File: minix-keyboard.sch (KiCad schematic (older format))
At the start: 126 parts, among them J1 AVR-ISP-6, SW1 SW_Push, U1 ATmega32U4-AU, U2 PRTR5V0U2X, Y1 16MHz

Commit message: Add promicro header
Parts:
- added U3: ProMicro-keebio, Keebio-Parts:ArduinoProMicro-TopSide, symbol cookpad-pad-rescue:ProMicro-keebio
- MX1, MX10, MX11, MX12, MX13, MX14, MX15, MX16, MX17, MX18, MX19, MX2, MX20, MX21, MX22, MX23, MX24, MX25, MX26, MX27, MX28, MX29, MX3, MX30, MX31, MX32, MX33, MX34, MX35, MX36, MX37, MX38, MX39, MX4, MX40, MX41, MX42, MX43, MX44, MX45, MX46, MX47, MX48, MX49, MX5, MX50, MX51, MX52, MX53, MX6, MX7, MX8, MX9: symbol MX_Alps_Hybrid:MX-NoLED -> minix-keyboard-rescue:MX-NoLED-MX_Alps_Hybrid
- U2: symbol random-keyboard-parts:PRTR5V0U2X -> minix-keyboard-rescue:PRTR5V0U2X-random-keyboard-parts
- USB1: symbol Type-C:HRO-TYPE-C-31-M-12 -> minix-keyboard-rescue:HRO-TYPE-C-31-M-12-Type-C
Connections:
- net MISO is gone; now on net COL10: J1.1 (MISO), U1.11 (PB3)
- net MOSI is gone; now on net COL11: J1.4 (MOSI), U1.10 (PB2)
- net SCK is gone; now on net COL9: J1.3 (SCK), U1.9 (PB1)
- net COL0: now also U1.25 (PD4), U3.7 (4/PD4)
- net COL1: now also U1.31 (PC6), U3.8 (5/PC6)
- net COL10: now also U3.15 (14/PB3)
- net COL11: now also U3.14 (16/PB2)
- net COL12: now also U1.30 (PB6), U3.13 (10/PB6)
- net COL2: now also U1.27 (PD7), U3.9 (6/PD7)
- net COL3: now also U1.1 (PE6), U3.10 (7/PE6)
- net COL4: now also U1.28 (PB4), U3.11 (8/PB4)
- net COL5: now also U1.29 (PB5), U3.12 (9/PB5)
- net COL6: now also U1.38 (PF5), U3.19 (A2/PF5)
- net COL7: now also U1.37 (PF6), U3.18 (A1/PF6)
- net COL8: now also U1.36 (PF7), U3.17 (A0/PF7)
- net COL9: now also U3.16 (15/PB1)
- net ROW0: now also U1.18 (PD0), U3.6 (3/PD0)
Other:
- note added: "ProMicro"

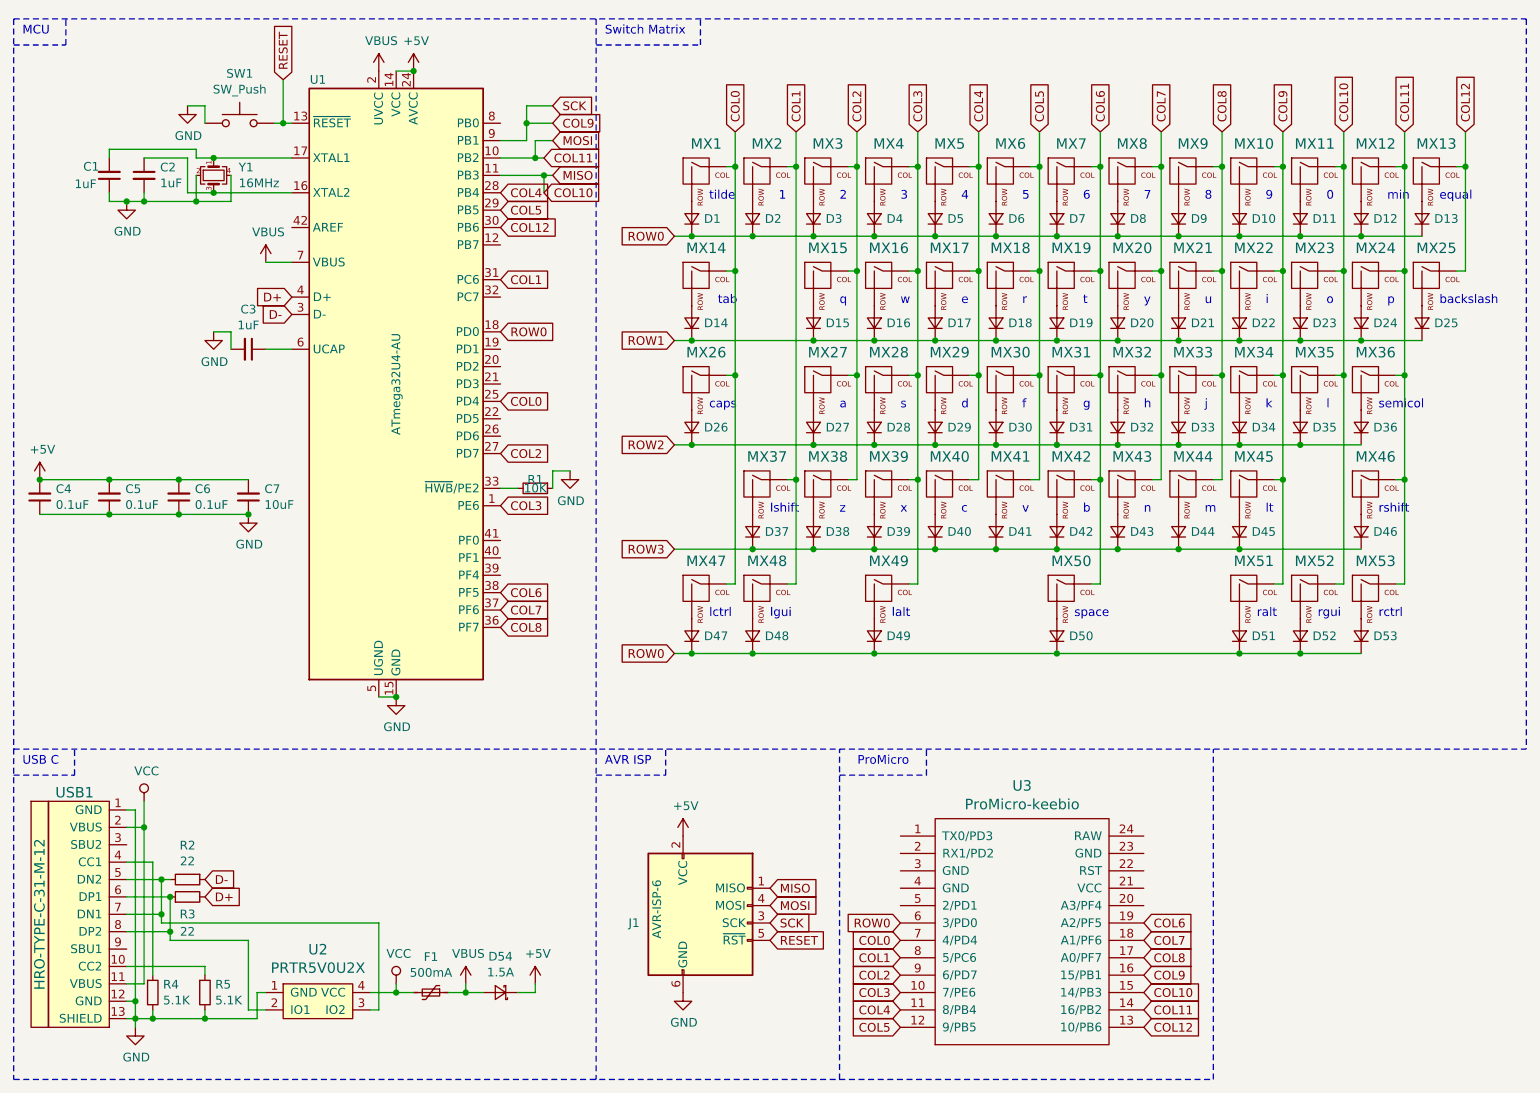
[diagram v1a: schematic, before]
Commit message: Update schematic
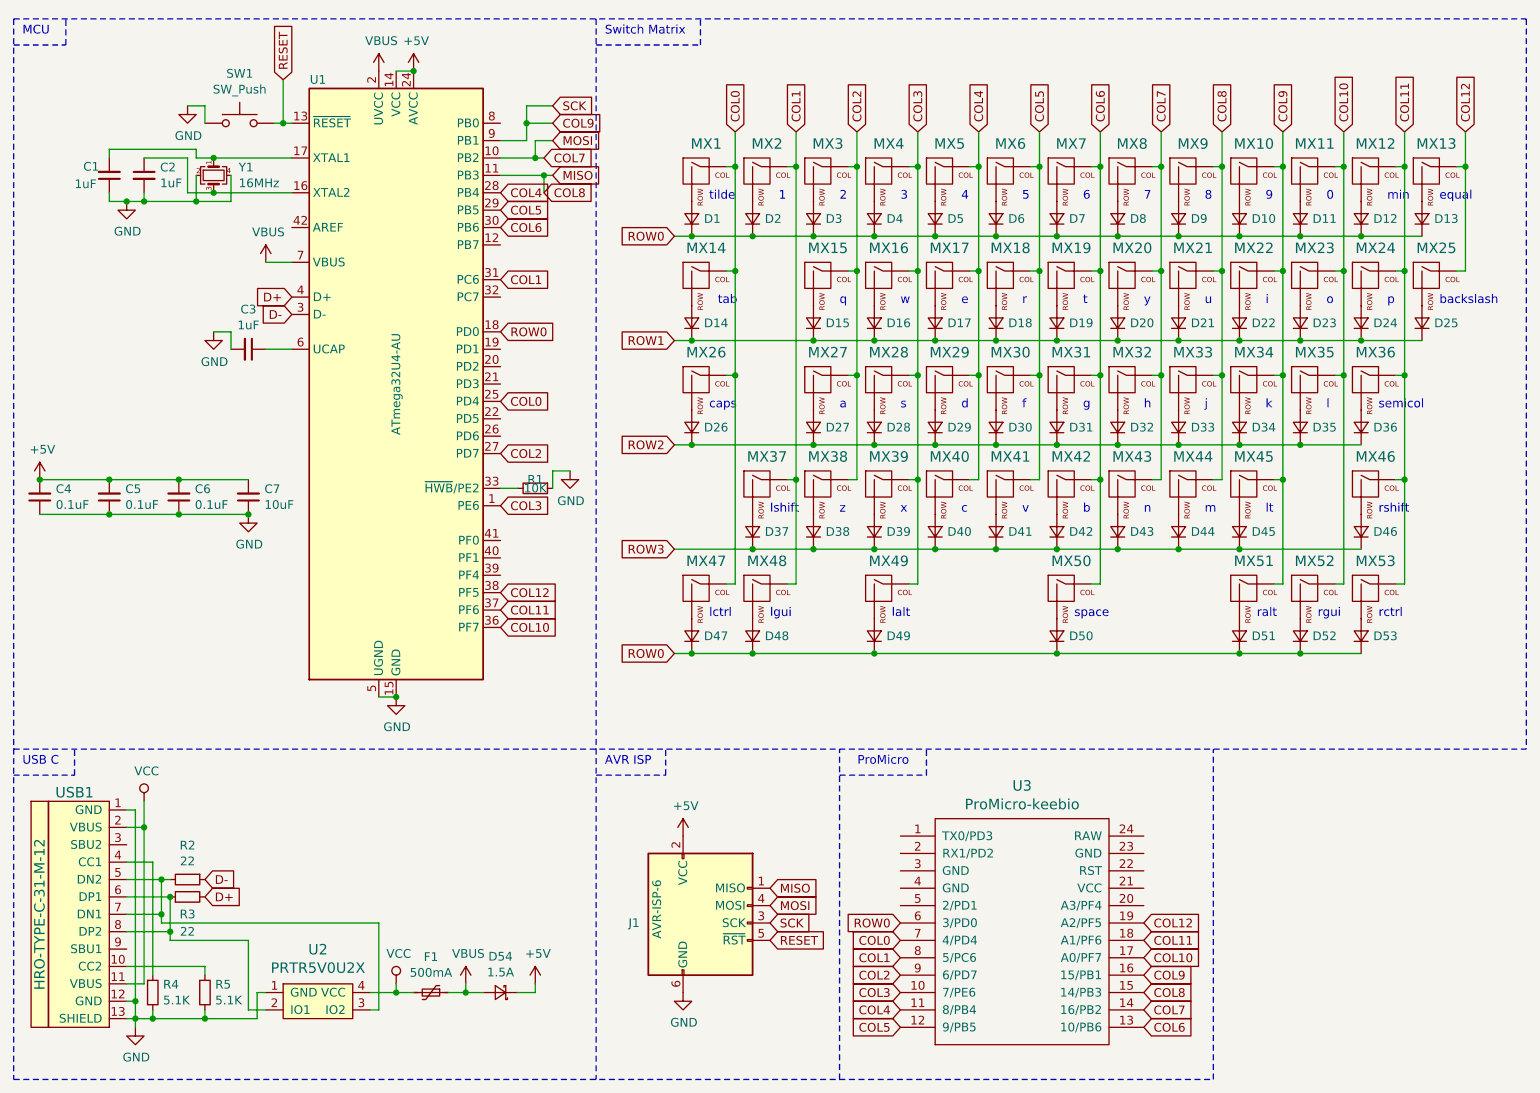
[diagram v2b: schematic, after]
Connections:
- net COL10: now also U1.36 (PF7), U3.17 (A0/PF7); no longer J1.1 (MISO), U1.11 (PB3), U3.15 (14/PB3)
- net COL11: now also U1.37 (PF6), U3.18 (A1/PF6); no longer J1.4 (MOSI), U1.10 (PB2), U3.14 (16/PB2)
- net COL12: now also U1.38 (PF5), U3.19 (A2/PF5); no longer U1.30 (PB6), U3.13 (10/PB6)
- net COL6: now also U1.30 (PB6), U3.13 (10/PB6); no longer U1.38 (PF5), U3.19 (A2/PF5)
- net COL7: now also J1.4 (MOSI), U1.10 (PB2), U3.14 (16/PB2); no longer U1.37 (PF6), U3.18 (A1/PF6)
- net COL8: now also J1.1 (MISO), U1.11 (PB3), U3.15 (14/PB3); no longer U1.36 (PF7), U3.17 (A0/PF7)
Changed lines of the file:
@@
 Text GLabel 3300 3300 2    50   Input ~ 0
 COL3
-Text GLabel 7000 5700 2    50   Input ~ 0
+Text GLabel 7000 6300 2    50   Input ~ 0
 COL6
-Text GLabel 7000 5800 2    50   Input ~ 0
+Text GLabel 7000 6200 2    50   Input ~ 0
 COL7
-Text GLabel 7000 5900 2    50   Input ~ 0
+Text GLabel 7000 6100 2    50   Input ~ 0
 COL8
 Text GLabel 7000 6000 2    50   Input ~ 0
 COL9
-Text GLabel 7000 6100 2    50   Input ~ 0
+Text GLabel 7000 5900 2    50   Input ~ 0
 COL10
-Text GLabel 7000 6200 2    50   Input ~ 0
+Text GLabel 7000 5800 2    50   Input ~ 0
 COL11
-Text GLabel 7000 6300 2    50   Input ~ 0
+Text GLabel 7000 5700 2    50   Input ~ 0
 COL12
-Text GLabel 3300 3800 2    50   Input ~ 0
+Text GLabel 3300 1700 2    50   Input ~ 0
 COL6
-Text GLabel 3300 3900 2    50   Input ~ 0
+Text GLabel 3550 1300 2    50   Input ~ 0
 COL7
-Text GLabel 3300 4000 2    50   Input ~ 0
+Text GLabel 3550 1500 2    50   Input ~ 0
 COL8
 Text GLabel 3600 1100 2    50   Input ~ 0
@@
 Wire Wire Line
 	3300 1200 3450 1200
-Text GLabel 3550 1500 2    50   Input ~ 0
+Text GLabel 3300 4000 2    50   Input ~ 0
 COL10
-Text GLabel 3550 1300 2    50   Input ~ 0
+Text GLabel 3300 3900 2    50   Input ~ 0
 COL11
-Text GLabel 3300 1700 2    50   Input ~ 0
+Text GLabel 3300 3800 2    50   Input ~ 0
 COL12
 Wire Wire Line
